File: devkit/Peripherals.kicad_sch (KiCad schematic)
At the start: 50 parts, among them IC501 APDS-9306-065, IC502 BMI270, IC503 LIS2MDLTR, IC504 BMP581, IC505 DRV2603RUNT, IC506 PCA9306JK, IC507 RV-8263-C8, J501 Jumper, J502 Jumper, J503 Jumper, J504 Jumper, J505 Jumper, J506 Jumper, J507 Jumper, M501 Vibrator DC Motor, X501 Current, X502 I2S, X503 Current, X504 I2C, X505 Current, X506 Current, X507 Current, X508 Current, X509 Motor, X510 Current

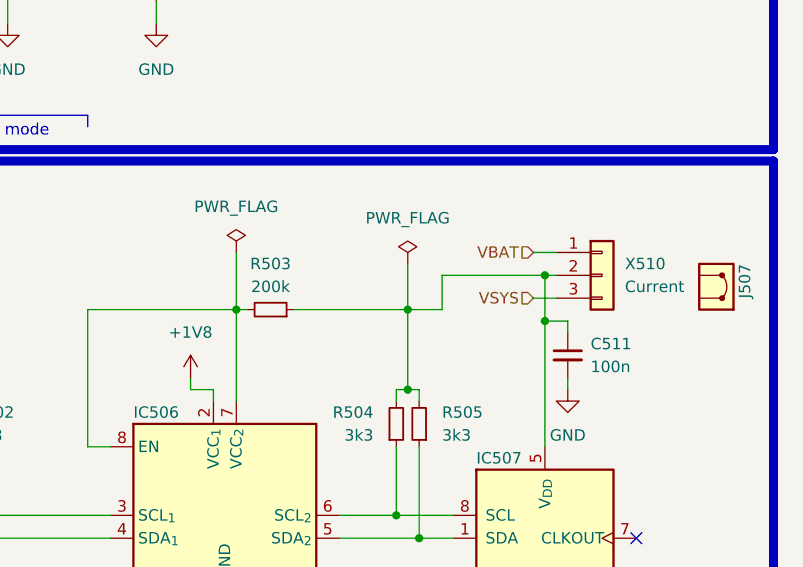
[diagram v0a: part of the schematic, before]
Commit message: Revert "Feature: Issue #186"
This reverts commit 73512b60dac517a3d61ff56758c38d705b52f64d.
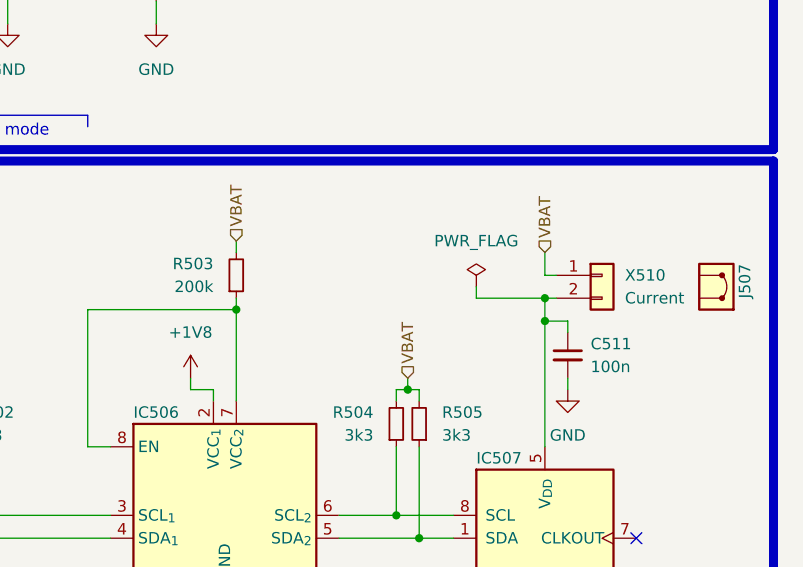
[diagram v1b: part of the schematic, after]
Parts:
- X510: footprint Connector_PinHeader_2.54mm:PinHeader_1x03_P2.54mm_Vertical -> Connector_PinHeader_2.54mm:PinHeader_1x02_P2.54mm_Vertical; symbol Connector_Generic:Conn_01x03 -> Connector_Generic:Conn_01x02; manf# 77311-818-03LF -> 77311-818-02LF; mouser# 649-77311-818-03LF -> 649-77311-818-02LF
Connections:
- net VBAT: now also R503.2, R504.2, R505.2
- net VSYS: no longer X510.3 (Pin_3)
- net at C511.1, IC507.5 (V_{DD}), X510.2 (Pin_2): no longer R503.1, R504.2, R505.2
- net at IC506.7 (VCC_{2}), IC506.8 (EN): now also R503.1; no longer R503.2
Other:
- moved on the sheet: R503
